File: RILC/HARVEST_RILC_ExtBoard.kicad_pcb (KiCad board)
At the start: 2 copper layers, 55 x 30 mm, 47 parts, among them J3 Conn_01x02, SW1 SW_SPST, SW2 SW_DIP_x04, U1 TPS92612DBVR, U2 TPS92612DBVR, U3 TPS92612DBVR, U4 TPS92612DBVR

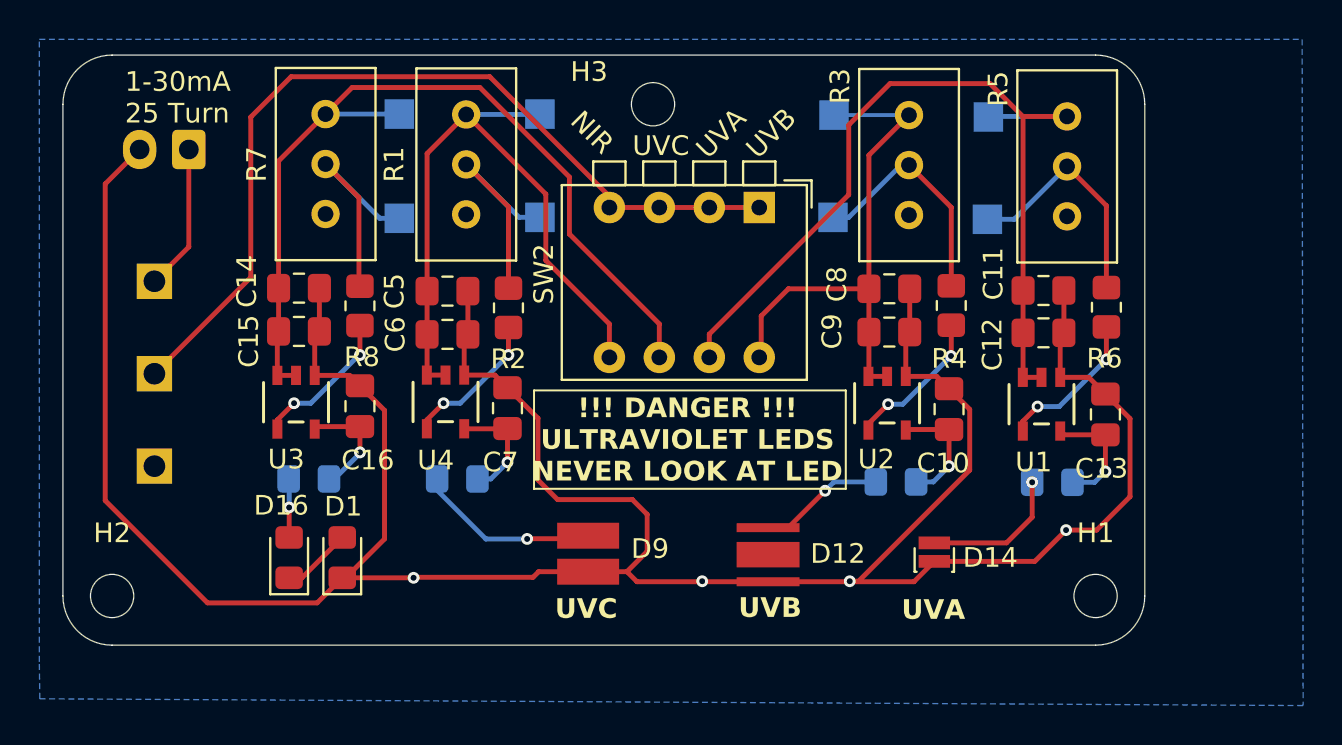
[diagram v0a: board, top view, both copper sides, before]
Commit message: V2.0: Produced Version
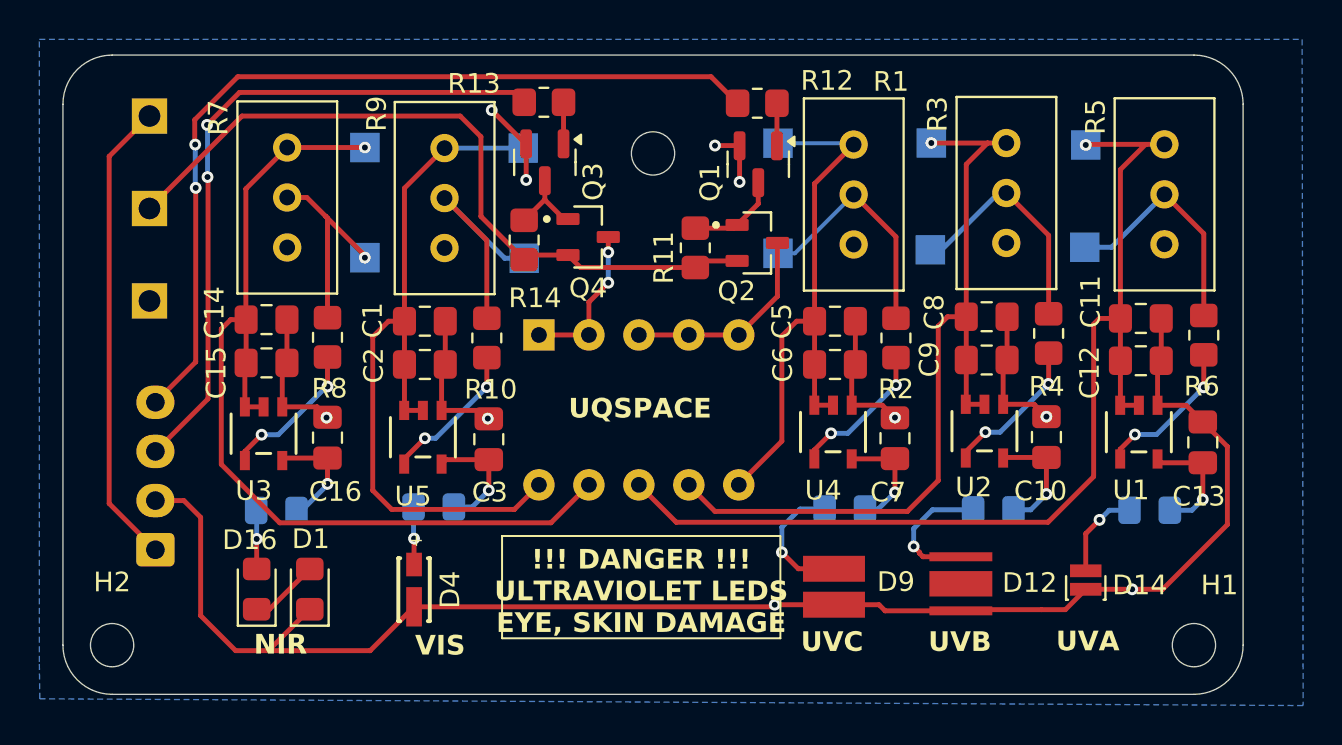
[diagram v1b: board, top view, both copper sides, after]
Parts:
- removed J3: Conn_01x02, Connector_JST:JST_XH_B2B-XH-A_1x02_P2.50mm_Vertical
- removed SW2: SW_DIP_x04, Button_Switch_THT:SW_DIP_SPSTx04_Piano_CTS_Series194-4MSTN_W7.62mm_P2.54mm
- added C1: 1u, Capacitor_SMD:C_0805_2012Metric_Pad1.18x1.45mm_HandSolder, F.Cu at (118.4, 43.5)
- added C2: 100n, Capacitor_SMD:C_0805_2012Metric_Pad1.18x1.45mm_HandSolder, F.Cu at (118.4, 45.7)
- added C3: 10n, Capacitor_SMD:C_0805_2012Metric_Pad1.18x1.45mm_HandSolder, F.Cu at (121.7, 49.5)
- added D2: CH_EN_LED_VIS, LED_SMD:LED_0805_2012Metric_Pad1.15x1.40mm_HandSolder, B.Cu at (118.8, 53.0)
- added D4: VIS1, 158301240_LED:WL-SWTP_3014, F.Cu at (117.8, 57.2)
- added J1: IN, Connector_JST:JST_XH_B4B-XH-A_1x04_P2.50mm_Vertical, B.Cu at (104.7, 55.1)
- added Q1: MMBT3904, Package_TO_SOT_SMD:SOT-23, F.Cu at (135.3, 35.5)
- added Q2: PMOS, DMG2305UX-7_Snapeda:SOT91P240X110-3N_DMG2305UX-7, F.Cu at (135.3, 39.5)
- added Q3: MMBT3904, Package_TO_SOT_SMD:SOT-23, F.Cu at (124.5, 35.5)
- added Q4: PMOS, DMG2305UX-7_Snapeda:SOT91P240X110-3N_DMG2305UX-7, F.Cu at (126.7, 39.2)
- added R10: 3.3, Resistor_SMD:R_0805_2012Metric_Pad1.20x1.40mm_HandSolder, F.Cu at (121.5, 44.4)
- added R11: 10k, Resistor_SMD:R_0805_2012Metric_Pad1.20x1.40mm_HandSolder, F.Cu at (132.2, 39.8)
- added R12: 10k, Resistor_SMD:R_0805_2012Metric_Pad1.20x1.40mm_HandSolder, F.Cu at (135.3, 32.5)
- added R13: 10k, Resistor_SMD:R_0805_2012Metric_Pad1.20x1.40mm_HandSolder, F.Cu at (124.5, 32.4)
- added R14: 10k, Resistor_SMD:R_0805_2012Metric_Pad1.20x1.40mm_HandSolder, F.Cu at (123.4, 39.4)
- added R9: Iset_100_Pot, Potentiometer_THT:Potentiometer_Bourns_3296W_Vertical, F.Cu at (119.4, 34.7)
- added SW3: SW_DIP_x05, Button_Switch_THT:SW_DIP_SPSTx05_Piano_CTS_Series194-5MSTN_W7.62mm_P2.54mm, B.Cu at (124.2, 44.2)
- added TP10: Pot-, TestPoint:TestPoint_Pad_1.5x1.5mm, B.Cu at (123.5, 40.3)
- added TP9: Pot+, TestPoint:TestPoint_Pad_1.5x1.5mm, B.Cu at (123.4, 34.7)
- added U5: TPS92612DBVR, TPS92612:SOT_12DBVR_TEX, F.Cu at (118.3, 49.4)
- moved C7 19.8 mm to (142.3, 49.5)
- moved C5 19.8 mm to (139.2, 43.5)
- moved D10 19.8 mm to (139.8, 53.1)
- moved C6 19.8 mm to (139.2, 45.7)
- moved R2 19.8 mm to (142.3, 44.4)
- moved U4 19.8 mm to (139.1, 49.2)
- moved R1 19.8 mm to (140.2, 34.5)
- moved D9 12.6 mm to (139.2, 57.0)
- moved TP4 12.2 mm to (136.3, 40.1)
- moved TP3 12.2 mm to (136.3, 34.5)
- moved D12 9.91 mm to (145.7, 56.9)
- moved SW1 8.40 mm to (104.4, 33.1)
- moved D14 7.83 mm to (152.0, 56.7)
- moved H1 5.59 mm to (157.5, 60.0)
- moved TP7 5.22 mm to (144.1, 39.9)
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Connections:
- SW1 pad 2: Net-(SW1-B) -> VIN
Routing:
- net Net-(SW1-B): track 45.0 -> 0.00 mm
- net /UV_EN: track 0.00 -> 44.3 mm, vias 0 -> 2
- net VIS_DRIV_PWR: track 0.00 -> 38.2 mm
- net VIN: track 0.00 -> 37.7 mm
- net /VIS_NIR_EN: track 0.00 -> 34.7 mm, vias 0 -> 2
- net GND: track 148.5 -> 114.9 mm, vias 4 -> 10
- net Net-(J1-Pin_1): track 7.42 -> 23.9 mm
- net UVB_DRIV_PWR: track 27.0 -> 41.8 mm, vias 0 -> 1
- net Net-(R10-Pad1): track 0.00 -> 12.3 mm
- net UVLED_PWR: track 0.00 -> 10.6 mm
- net VIS_NIR_LED_PWR: track 0.00 -> 7.93 mm, vias 0 -> 2
- net Net-(U5-IN): track 0.00 -> 7.48 mm, vias 0 -> 2
- net UVA_DRIV_PWR: track 45.7 -> 52.9 mm, vias 0 -> 1
- net Net-(D2-A): track 0.00 -> 6.18 mm, vias 0 -> 1
- net UVC_DRIV_PWR: track 34.1 -> 29.3 mm
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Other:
- board size 55 x 30 mm -> 60 x 32.5 mm
- board text added: "!!! DANGER !!! ULTRAVIOLET LEDS EYE, SKIN DAMAGE"
- board text added: "ON"
- board text added: "Pot+"
- board text added: "Pot-"
- board text added: "R.I.L.C V2.0 THESEUS 2026 Y.BHALLA"
- board text added: "RATING Current: 1-30mA 25 Turn Pot"
- board text added: "UQSPACE"
- board text added: "VIS"
- board text added: "VIS ON"
- board text removed: "!!! DANGER !!! ULTRAVIOLET LEDS NEVER LOOK AT LED"
- board text removed: "1-30mA 25 Turn"
- board text removed: "EXTREME DANGER TO EYE, SKIN."
- board text removed: "RILC PCB POC V1.1 UQS | PAYL | THESEUS 2026 Y.BHALLA"
- board text removed: "UVA"
- board text removed: "UVB"
- board text removed: "UVC"
